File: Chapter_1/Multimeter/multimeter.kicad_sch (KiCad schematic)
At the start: 28 parts, among them Q1 BC557, Q10 BC557, Q11 BC557, Q12 BC557, Q13 BC557, Q14 IRLZ44N, Q15 BC557, Q16 BC557, Q2 BC557, Q21 IRLZ44N, Q3 BC557, Q4 BC557, Q5 BC557, Q6 BC557, Q7 BC557, Q8 BC557, Q9 BC557, SW1-AMMTER1 SW_Push, SW2-VOLTMETER1 SW_Push, SW4 SW_Push

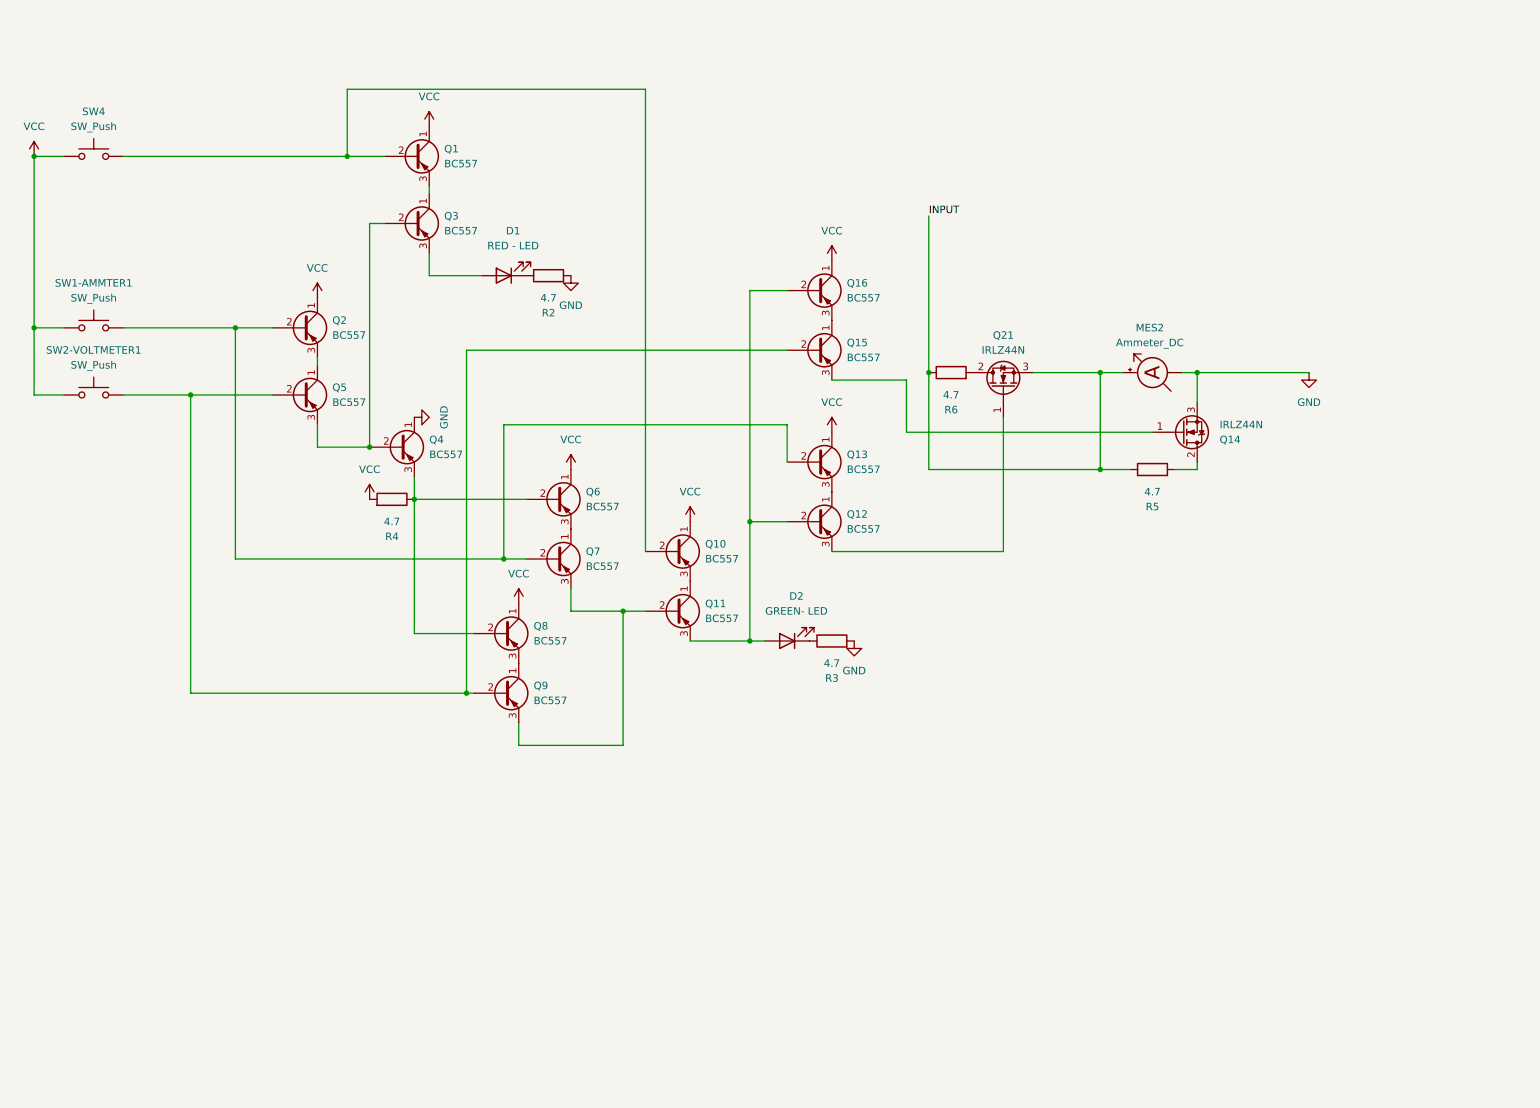
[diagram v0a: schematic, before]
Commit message: Corrected design
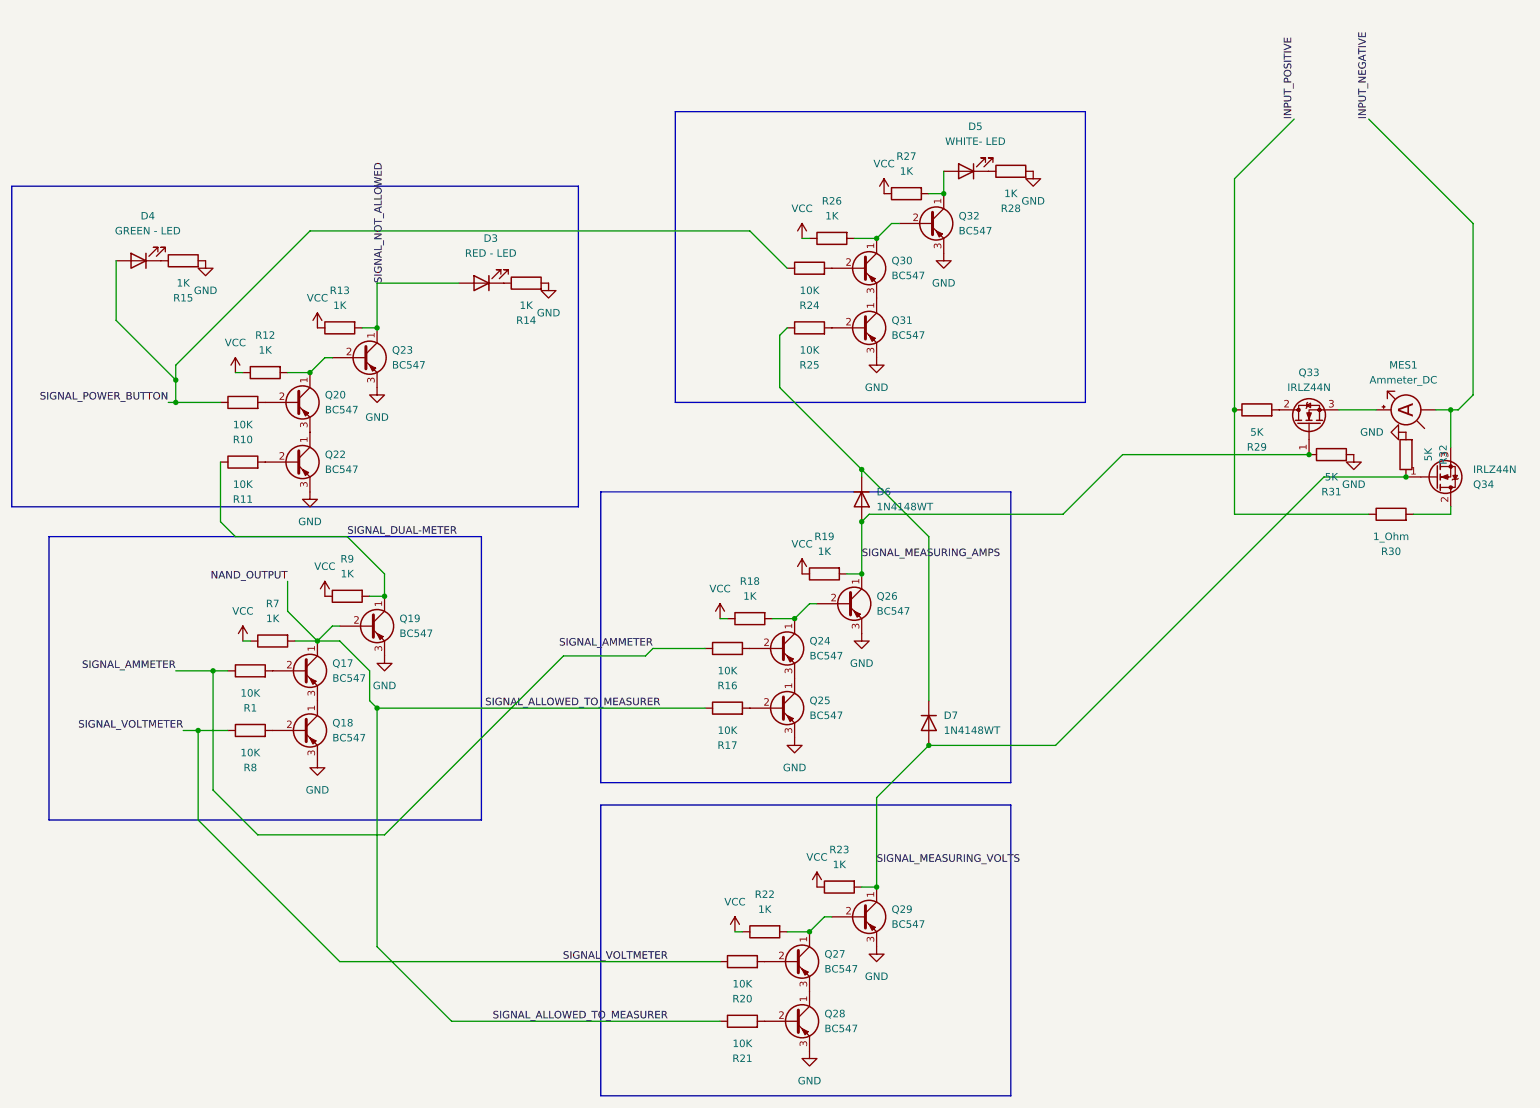
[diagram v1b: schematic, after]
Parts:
- removed D1: RED - LED, symbol Device:LED
- removed D2: GREEN- LED, symbol Device:LED
- removed MES2: Ammeter_DC, symbol Device:Ammeter_DC
- removed Q1, Q10, Q11, Q12, Q13, Q15, Q16, Q2, Q3, Q4, Q5, Q6, Q7, Q8, Q9: BC557, Package_TO_SOT_THT:TO-92_Inline, symbol Transistor_BJT:BC557
- removed Q14, Q21: IRLZ44N, Package_TO_SOT_THT:TO-220-3_Vertical, symbol Transistor_FET:IRLZ44N
- removed R2, R3, R4, R5, R6: 4.7, symbol Device:R
- removed SW1-AMMTER1, SW2-VOLTMETER1, SW4: SW_Push, symbol Switch:SW_Push
- added D3: RED - LED, symbol Device:LED
- added D4: GREEN - LED, symbol Device:LED
- added D5: WHITE- LED, symbol Device:LED
- added D6, D7: 1N4148WT, Diode_SMD:D_SOD-523, symbol Diode:1N4148WT
- added MES1: Ammeter_DC, symbol Device:Ammeter_DC
- added Q17, Q18, Q19, Q20, Q22, Q23, Q24, Q25, Q26, Q27, Q28, Q29, Q30, Q31, Q32: BC547, Package_TO_SOT_THT:TO-92_Inline, symbol Transistor_BJT:BC557
- added Q33, Q34: IRLZ44N, Package_TO_SOT_THT:TO-220-3_Vertical, symbol Transistor_FET:IRLZ44N
- added R1, R10, R11, R16, R17, R20, R21, R24, R25, R8: 10K, symbol Device:R
- added R12, R13, R14, R15, R18, R19, R22, R23, R26, R27, R28, R7, R9: 1K, symbol Device:R
- added R29, R31, R32: 5K, symbol Device:R
- added R30: 1_Ohm, symbol Device:R
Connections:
- net GND: now also Q18.3 (E), Q19.3 (E), Q22.3 (E), Q23.3 (E), Q25.3 (E), Q26.3 (E), Q28.3 (E), Q29.3 (E), Q31.3 (E), Q32.3 (E), R14.2, R15.2, R28.2, R31.2, R32.2
- net VCC: now also R12.1, R13.1, R18.1, R19.1, R22.1, R23.1, R26.1, R27.1, R7.1, R9.1
- new net: D5.2 (A), Q32.1 (C), R27.2
- new net: Q27.2 (B), R20.2
- new net: Q17.2 (B), R1.2
- new net: Q17.3 (E), Q18.1 (C)
- new net: Q20.3 (E), Q22.1 (C)
- new net: Q22.2 (B), R11.2
- new net: Q33.2 (D), R29.2
- new net: MES1.2 (+), Q33.3 (S)
- new net: D3.1 (K), R14.1
- new net: Q30.1 (C), Q32.2 (B), R26.2
- new net: Q18.2 (B), R8.2
- new net: Q27.3 (E), Q28.1 (C)
- new net: Q28.2 (B), R21.2
- new net: Q20.1 (C), Q23.2 (B), R12.2
- new net: Q20.2 (B), R10.2
- new net: Q34.2 (D), R30.2
- new net: D4.1 (K), R15.1
- new net: Q27.1 (C), Q29.2 (B), R22.2
- new net: D5.1 (K), R28.1
- new net: Q24.1 (C), Q26.2 (B), R18.2
- new net: Q24.2 (B), R16.2
- new net: Q24.3 (E), Q25.1 (C)
- new net: Q30.2 (B), R24.2
- new net: Q30.3 (E), Q31.1 (C)
- new net: D6.1 (K), D7.1 (K), R25.1
- new net: Q31.2 (B), R25.2
- new net: Q25.2 (B), R17.2
- new net INPUT_NEGATIVE: MES1.1 (-), Q34.3 (S)
- new net INPUT_POSITIVE: R29.1, R30.1
- new net NAND_OUTPUT: Q17.1 (C), Q19.2 (B), R17.1, R21.1, R7.2
- new net SIGNAL_AMMETER: R1.1, R16.1
- new net SIGNAL_DUAL-METER: Q19.1 (C), R11.1, R9.2
- new net SIGNAL_MEASURING_AMPS: D6.2 (A), Q26.1 (C), Q33.1 (G), R19.2, R31.1
- new net SIGNAL_MEASURING_VOLTS: D7.2 (A), Q29.1 (C), Q34.1 (G), R23.2, R32.1
- new net SIGNAL_NOT_ALLOWED: D3.2 (A), Q23.1 (C), R13.2
- new net SIGNAL_POWER_BUTTON: D4.2 (A), R10.1, R24.1
- new net SIGNAL_VOLTMETER: R20.1, R8.1
